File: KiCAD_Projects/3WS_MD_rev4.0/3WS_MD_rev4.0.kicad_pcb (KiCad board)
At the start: 2 copper layers, 76 x 93 mm, 139 parts, among them P1 CONN_01X01, P11 TST, P12 TST, P13 CONN_01X06, P14 CONN_01X02, P15 CONN_01X02, P16 CONN_01X04, P17 CONN_01X04, P18 CONN_01X04, P19 CONN_01X04, P2 CONN_01X01, P20 CONN_01X06, P3 CONN_01X04, P4 CONN_02X02, P5 TST, P6 CONN_01X04, P7 CONN_01X02, P8 CONN_01X04, P9 TST, Q1 MOSFET_N, Q2 MOSFET_N, Q3 MOSFET_N, Q4 MOSFET_N, Q5 MOSFET_N, Q6 MOSFET_N, Q7 MOSFET_N, Q8 MOSFET_N, Q9 MOSFET_N, SW1 SW_PUSH, SW2 SW_PUSH, SW3 SW_PUSH, U1 STM32F103_48, U10 NCP1117ST33T3G, U2 SI8234, U3 SI8234, U4 LM7812, U5 SI8234, U6 SI8234, U7 NCP1117ST33T3G, U8 MAX3051, U9 SW_ROTARY_16, X2 CRYSTAL

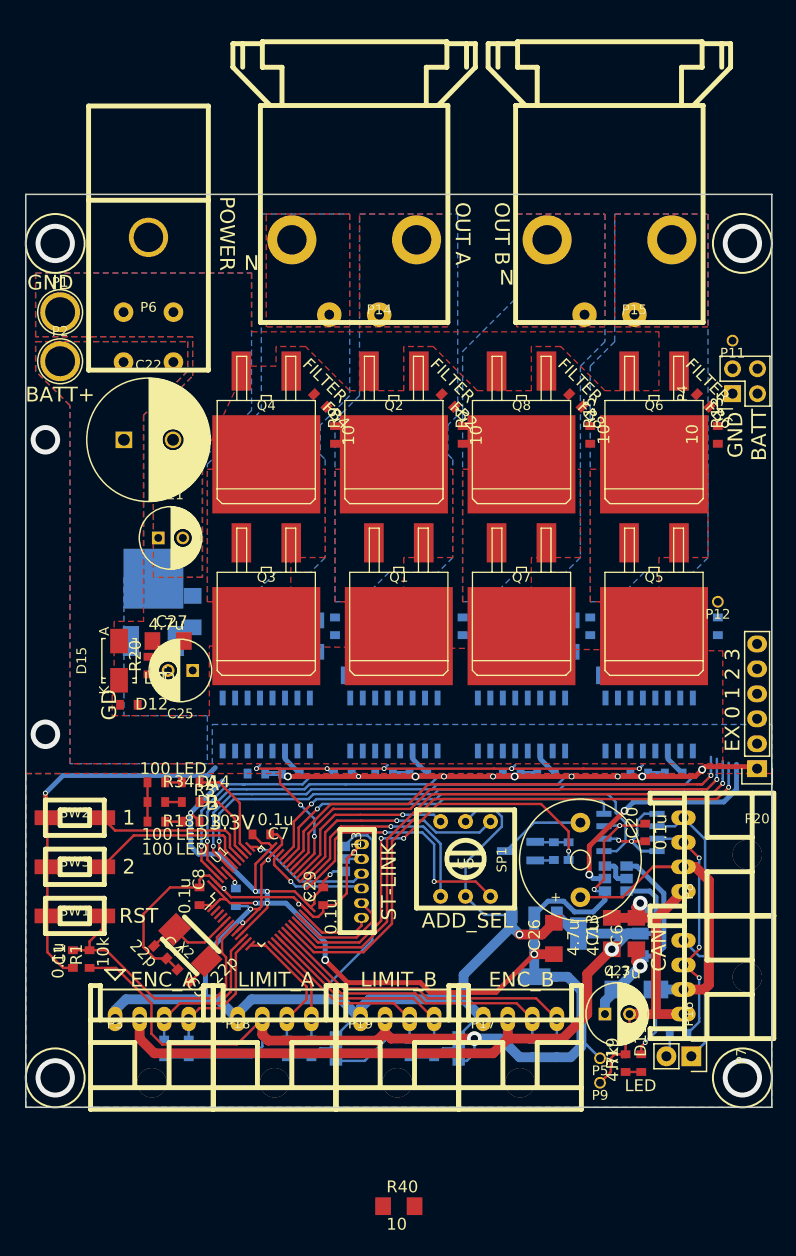
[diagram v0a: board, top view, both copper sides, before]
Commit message: no message
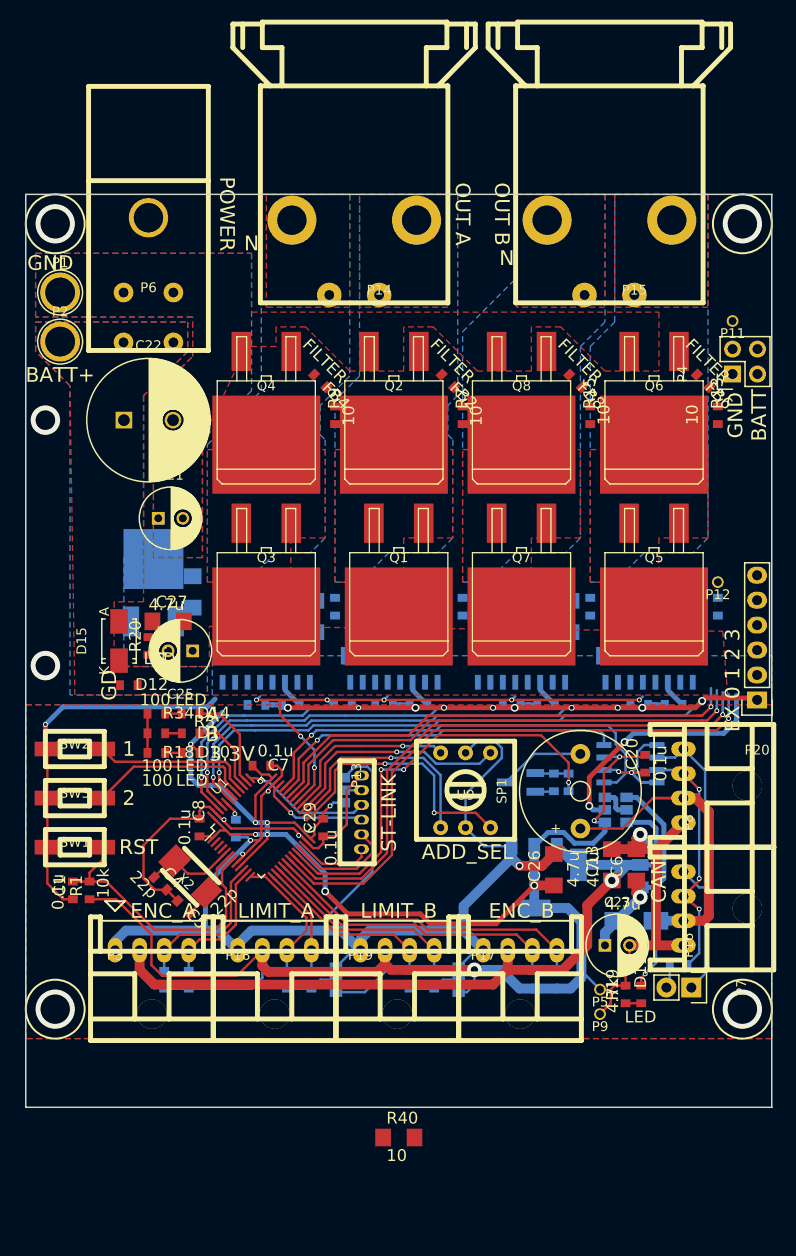
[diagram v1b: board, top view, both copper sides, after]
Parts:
- moved Q9 7.00 mm to (50.4, 59.9)
- moved R32 7.00 mm to (55.3, 59.9)
- moved R33 7.00 mm to (53.8, 59.9)
- moved C1 7.00 mm to (4.80, 70.9)
- moved C13 7.00 mm to (59.7, 68.3)
- moved C14 7.00 mm to (66.0, 52.0)
- moved C15 7.00 mm to (53.0, 52.0)
- moved C2 7.00 mm to (40.0, 52.0)
- moved C20 7.00 mm to (63.1, 58.0)
- moved C23 7.00 mm to (59.0, 76.5)
- moved C26 7.00 mm to (53.8, 68.8)
- moved C29 7.00 mm to (30.3, 64.5)
- moved C3 7.00 mm to (27.0, 52.0)
- moved C4 7.00 mm to (13.7, 70.2)
- moved C5 7.00 mm to (16.1, 72.6)
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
